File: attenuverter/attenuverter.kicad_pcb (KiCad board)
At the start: 2 copper layers, 71.9 x 168.7 mm, 89 parts, among them J1 Power, J10 Conn_01x03_Socket, J11 Output 1, J12 Input 1, J13 Conn_01x03_Socket, J14 Conn_01x03_Socket, J15 Output 1, J16 Input 1, J17 Conn_01x03_Socket, J18 Conn_01x03_Socket, J19 Output 1, J2 Power, J3 Power, J4 Input 1, J5 Conn_01x03_Socket, J6 Conn_01x03_Socket, J7 Output 1, J8 Input 1, J9 Conn_01x03_Socket, U1 TL074, U2 TL074, U3 TL074

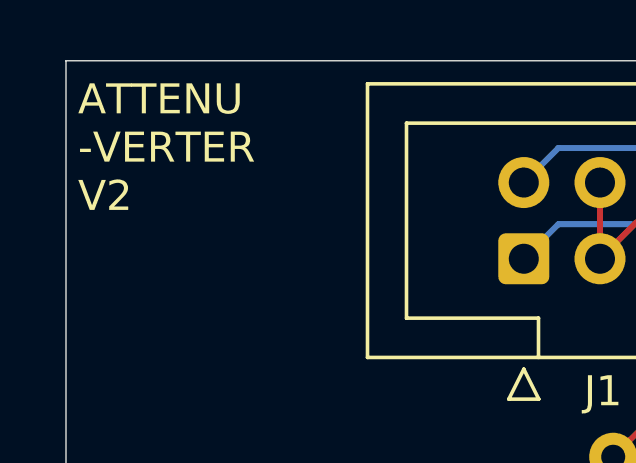
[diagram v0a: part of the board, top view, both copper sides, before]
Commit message: Vca fixes
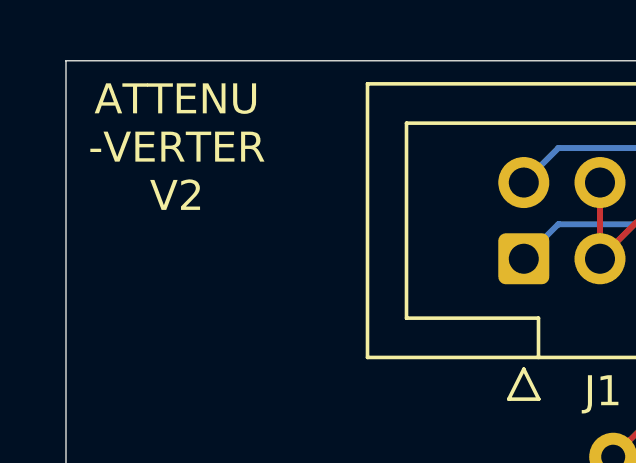
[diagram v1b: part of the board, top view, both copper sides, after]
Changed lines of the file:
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@@
 	)
 	(gr_text "ATTENU\n-VERTER\nV2"
-		(at 20.7 21 0)
+		(at 24 21 0)
 		(layer "F.SilkS")
 		(effects
@@
 				(thickness 0.15)
 			)
-			(justify left)
 		)
 	)
